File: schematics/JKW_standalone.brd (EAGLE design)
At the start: 159.4 x 80.7 mm, 217 parts, among them IC1 4093D, IC2 AT-MEGA-8L, IC4 ATMEGA2560-16AU, Q1 BSS84, Q10 BSS84, Q11 BSS84, Q2 BSS84, Q3 BSS84, Q4 BSS84, Q5 BSS84, Q6 BSS84, Q7 BSS84, Q8 BSS84, Q9 BSS84, T1 Mouser: 771-2N7002BK215 , N-C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, T10 Mouser: 771-2N7002BK215 , N-C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, T11 Mouser: 771-2N7002BK215 , N-C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, T12 Mouser: 771-2N7002BK215 , N-C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, T2 Mouser: 771-2N7002BK215 , N-C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, T3 Mouser: 771-2N7002BK215 , N-C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, T4 T-IRLMS6702, T5 Mouser: 771-2N7002BK215 , N-C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, T6 Mouser: 771-2N7002BK215 , N-C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, T7 Mouser: 771-2N7002BK215 , N-C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, T8 Mouser: 771-2N7002BK215 , N-C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, T9 Mouser: 771-2N7002BK215 , N-C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

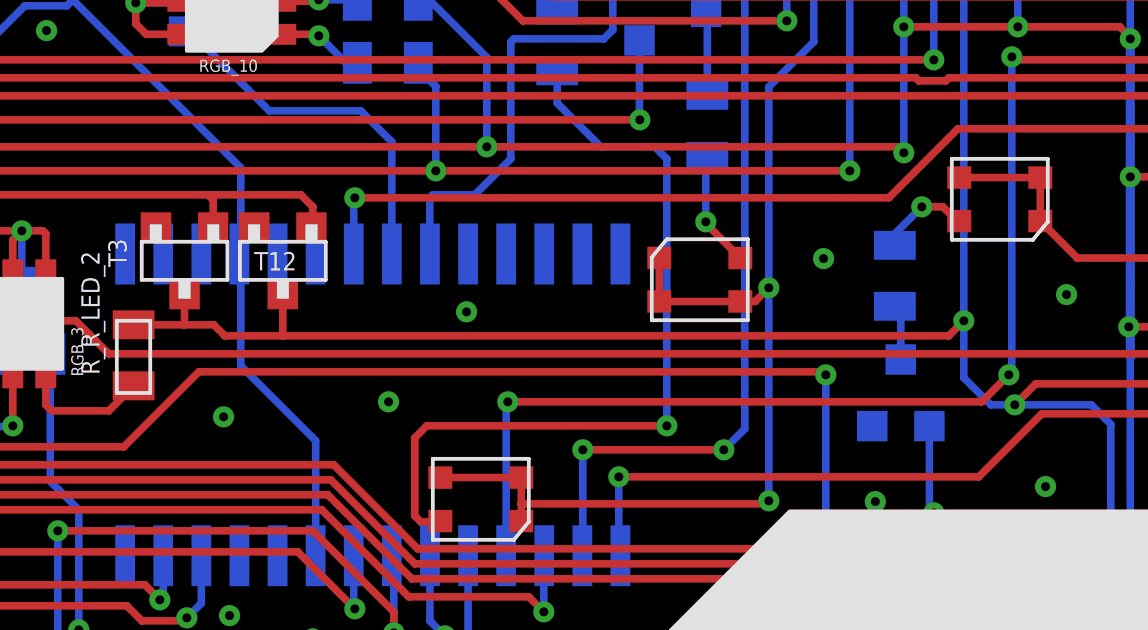
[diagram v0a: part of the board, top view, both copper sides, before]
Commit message: Improved schematic
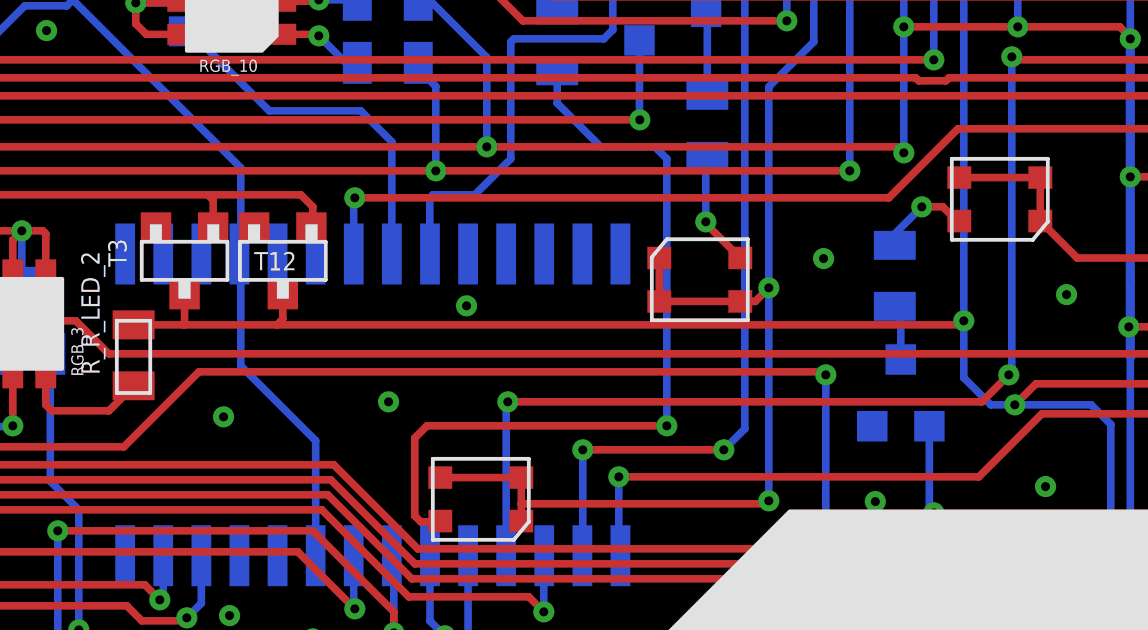
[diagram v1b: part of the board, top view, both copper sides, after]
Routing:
- net RED_INSTR: track 287.7 -> 287.1 mm
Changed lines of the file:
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@@
 <?xml version="1.0" encoding="utf-8"?>
 <!DOCTYPE eagle SYSTEM "eagle.dtd">
-<eagle version="6.1">
+<eagle version="6.2">
 <drawing>
 <settings>
@@
 <contactref element="D_P_MCCOI" pad="1"/>
 <via x="86.325" y="58.6" extent="1-16" drill="0.3"/>
-<via x="105.625" y="52" extent="1-16" drill="0.3"/>
+<via x="105.625" y="52.2" extent="1-16" drill="0.3"/>
 <via x="97.725" y="41.875" extent="1-16" drill="0.3"/>
 <via x="103.825" y="68.275" extent="1-16" drill="0.3"/>
@@
 <wire x1="146.884" y1="54" x2="146.984" y2="53.9" width="0.254" layer="1"/>
 <wire x1="94.525" y1="51.566" x2="96.2" y2="51.566" width="0.254" layer="1"/>
-<wire x1="96.2" y1="51.566" x2="97.2021" y2="51.566" width="0.254" layer="1"/>
-<wire x1="97.2021" y1="51.566" x2="97.5681" y2="51.2" width="0.254" layer="1"/>
-<wire x1="97.5681" y1="51.2" x2="99.5" y2="51.2" width="0.254" layer="1"/>
-<wire x1="99.5" y1="51.2" x2="121.7" y2="51.2" width="0.254" layer="1"/>
-<wire x1="121.7" y1="51.2" x2="122.2" y2="51.7" width="0.254" layer="1"/>
 <via x="122.2" y="51.7" extent="1-16" drill="0.3"/>
 <wire x1="96.225" y1="52.5889" x2="96.225" y2="51.591" width="0.254" layer="1"/>
 <wire x1="96.225" y1="51.591" x2="96.2" y2="51.566" width="0.254" layer="1"/>
-<wire x1="99.5" y1="52.5889" x2="99.5" y2="51.2" width="0.254" layer="1"/>
 <wire x1="122.2" y1="49.8" x2="123.1" y2="48.9" width="0.254" layer="16"/>
 <wire x1="123.1" y1="48.9" x2="123.9" y2="48.9" width="0.254" layer="16"/>
+<wire x1="96.2" y1="51.566" x2="99.3" y2="51.566" width="0.254" layer="1"/>
+<wire x1="99.3" y1="51.566" x2="122.066" y2="51.566" width="0.254" layer="1"/>
+<wire x1="122.066" y1="51.566" x2="122.2" y2="51.7" width="0.254" layer="1"/>
+<wire x1="99.5" y1="52.5889" x2="99.5" y2="51.766" width="0.254" layer="1"/>
+<wire x1="99.5" y1="51.766" x2="99.3" y2="51.566" width="0.254" layer="1"/>
 </signal>
 <signal name="N$70">
